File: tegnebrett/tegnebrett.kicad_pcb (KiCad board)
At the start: 6 copper layers, 195.2 x 101 mm, 204 parts, among them J1 FH12-45S-0.5SH55, J2 FH12-6S-1SH55, J3 Conn_ST_STDC14, J4 USB-A1HSW6, J5 MCU_Header_Pin, J6 FPGA_debug, J7 FPGA_Header_Pin, J8 DA15_Socket, J9 PJ-002A, SW1 SW_Push, SW2 SW_Push, SW3 MCU_Button, SW4 Reset, SW5 Undo, SW6 FPGA_Button, U1 STM32U5G7VJTxQ, U2 XC7A100T-2FTG256I, U3 Oscillator 100MHz, U4 IS66WVH16M8DBLL-100B1LI1, U5 VGA Transceiver, U6 VGA Transciever, U7 TPS54294PWP2, U8 TPS54294PWP1, Y1 48MHz

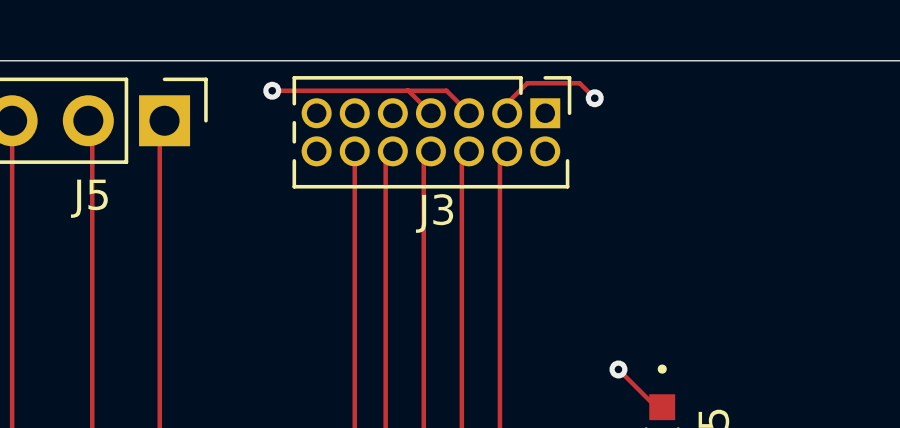
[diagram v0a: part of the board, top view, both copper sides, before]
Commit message: feat: PCB updates
Latest stuff from Tormod.
We still have 77 Errors and 2 warnings, but we'll ship this!
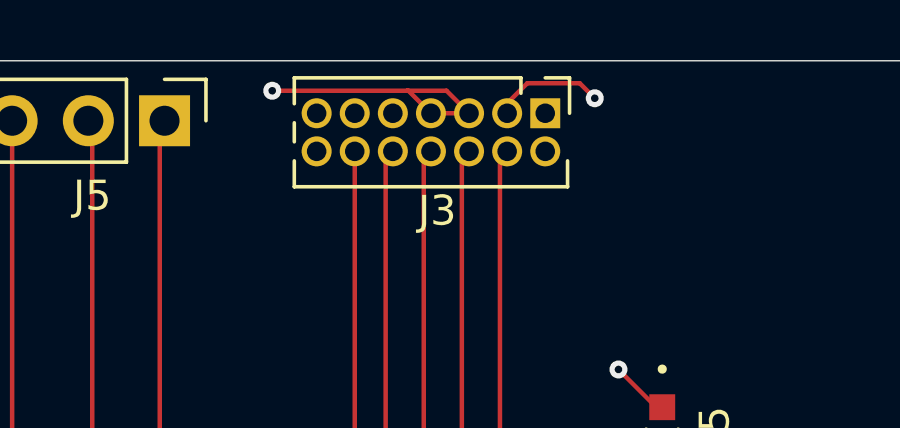
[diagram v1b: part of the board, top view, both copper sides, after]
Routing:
- net +3V3: track 1151.6 -> 420.5 mm
- net GND: track 612.8 -> 614.1 mm
- added copper zone on In4.Cu, net +3V3
